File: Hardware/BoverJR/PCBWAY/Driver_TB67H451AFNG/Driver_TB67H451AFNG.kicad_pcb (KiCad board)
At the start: 2 copper layers, 25 x 25 mm, 8 parts, among them J1 POWER, J3 MOTOR, J4 Conn_01x04_Pin, U1 TB67H451AFNG

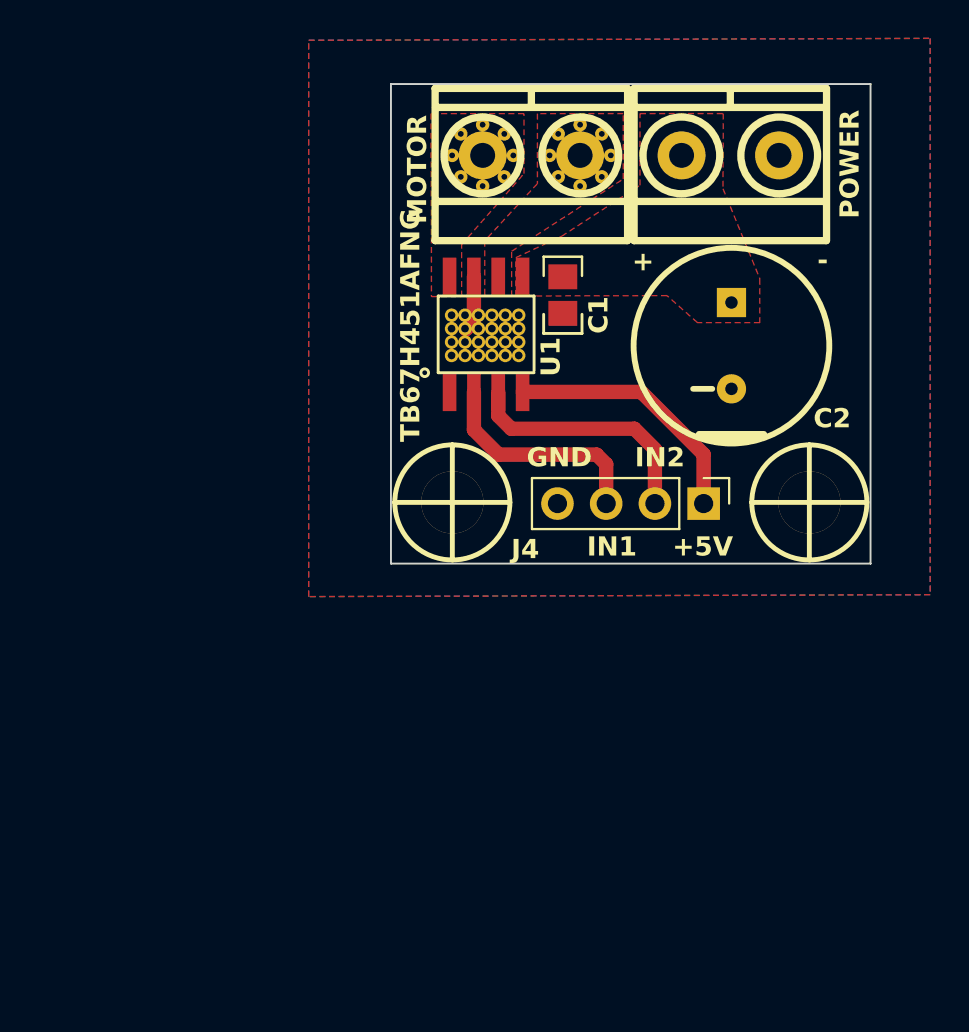
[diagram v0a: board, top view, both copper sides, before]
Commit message: cambios gerber
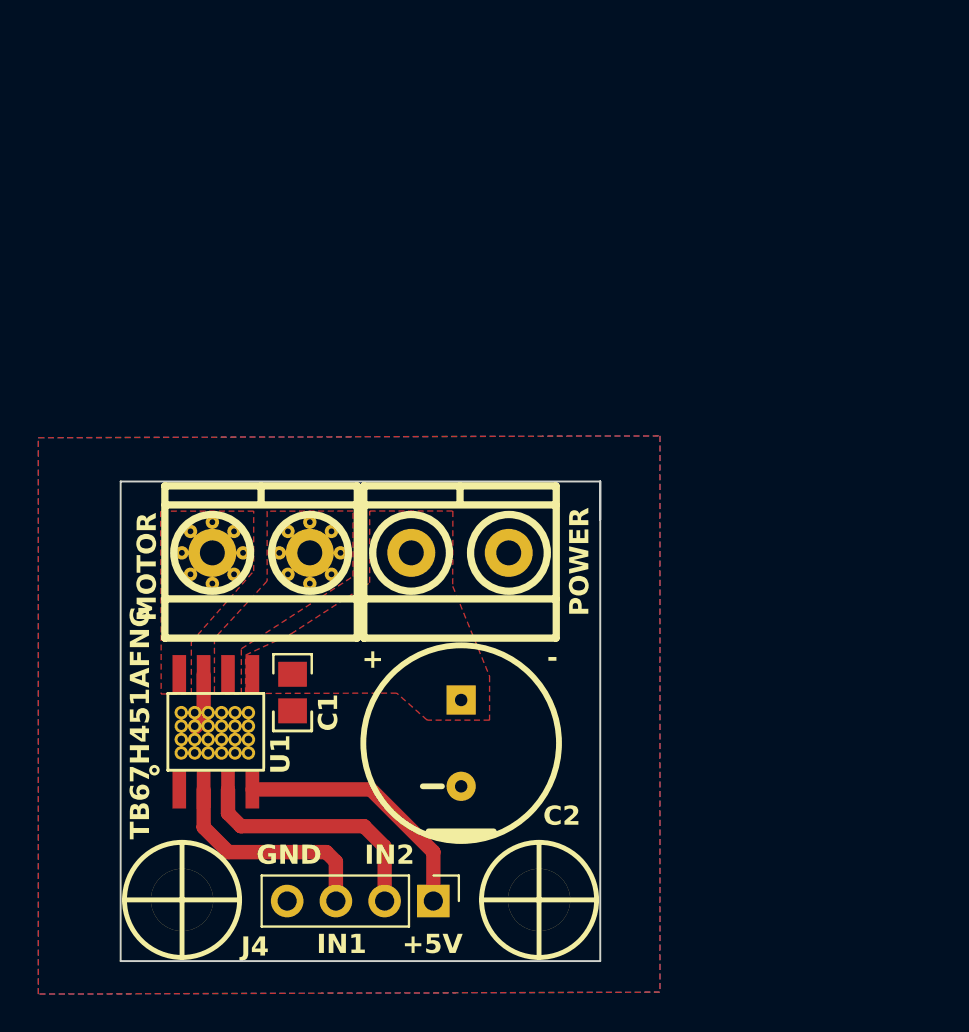
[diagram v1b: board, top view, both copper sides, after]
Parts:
- moved C1 25.1 mm to (140.2, 118.0)
- moved C2 25.1 mm to (148.9, 120.6)
- moved H1 25.1 mm to (134.4, 128.8)
- moved H2 25.1 mm to (153.0, 128.8)
- moved J1 25.1 mm to (148.9, 110.7)
- moved J3 25.1 mm to (138.5, 110.7)
- moved J4 25.1 mm to (147.5, 128.9)
- moved U1 25.1 mm to (136.2, 120.0)
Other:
- outline, holes or cut-outs redrawn
